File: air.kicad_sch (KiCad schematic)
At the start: 36 parts, among them J1 Conn_01x05, J2 Conn_01x05, J3 Conn_01x04, U1 MT9700, U2 AIR32F103CBT6-LQFP48, U3 RT9013-33GB, U4 USBLC6-2SC6, Y1 8M/20pF

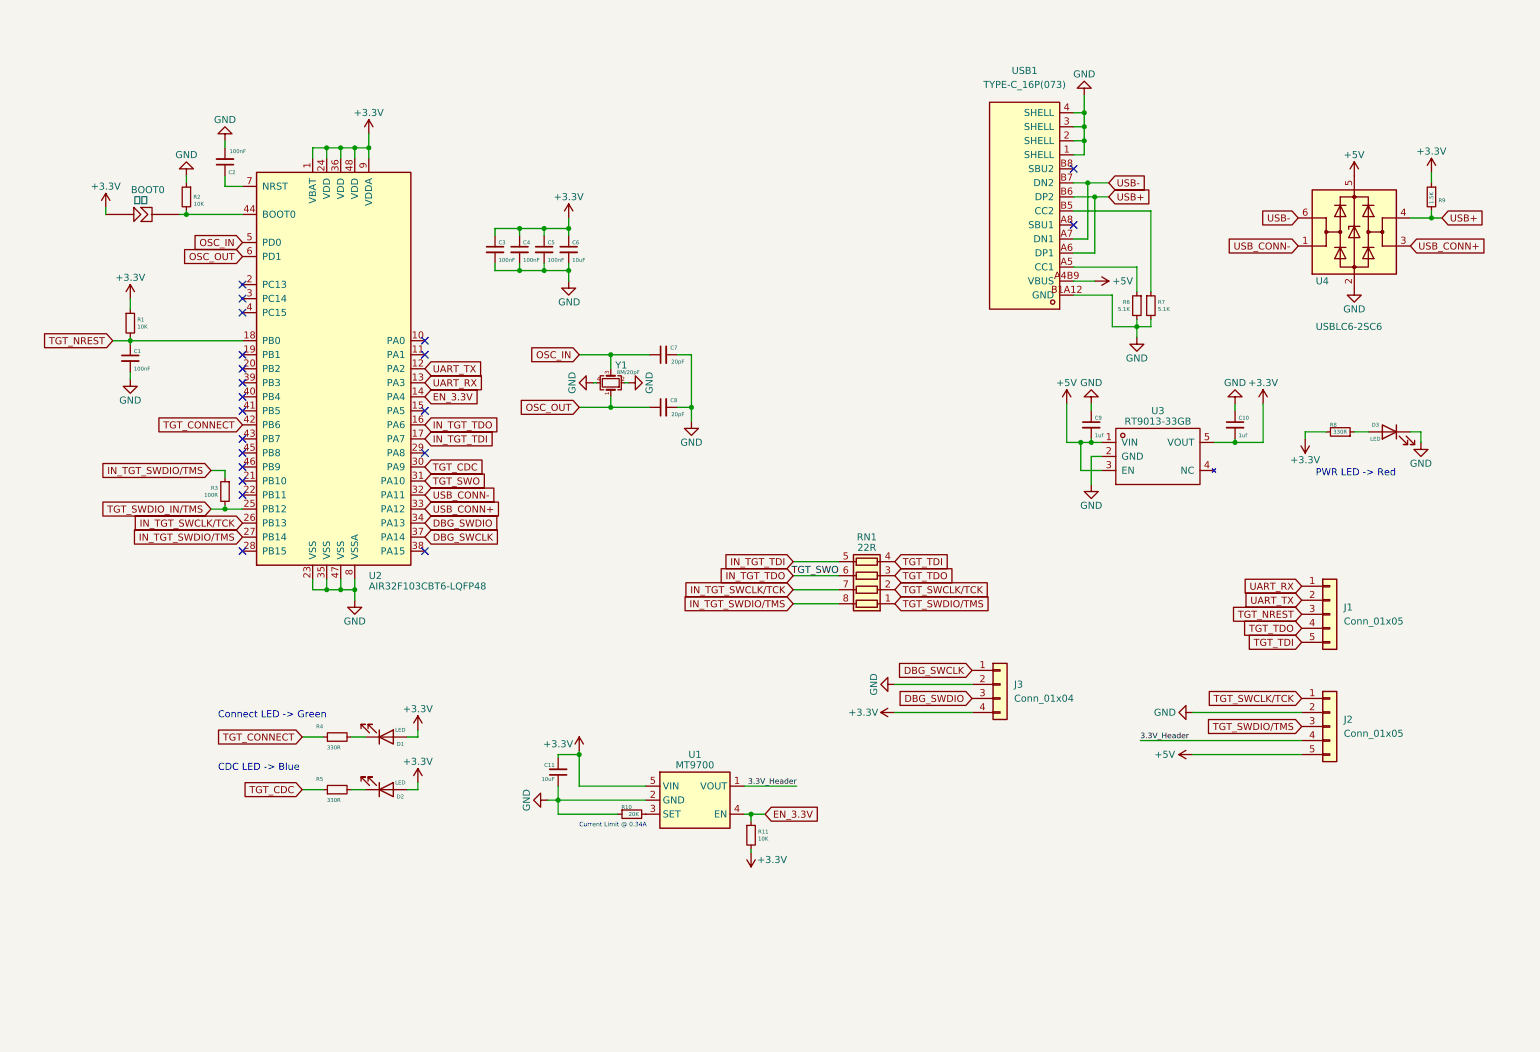
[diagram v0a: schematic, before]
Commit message: still 1.6 but contain some fix to publish work
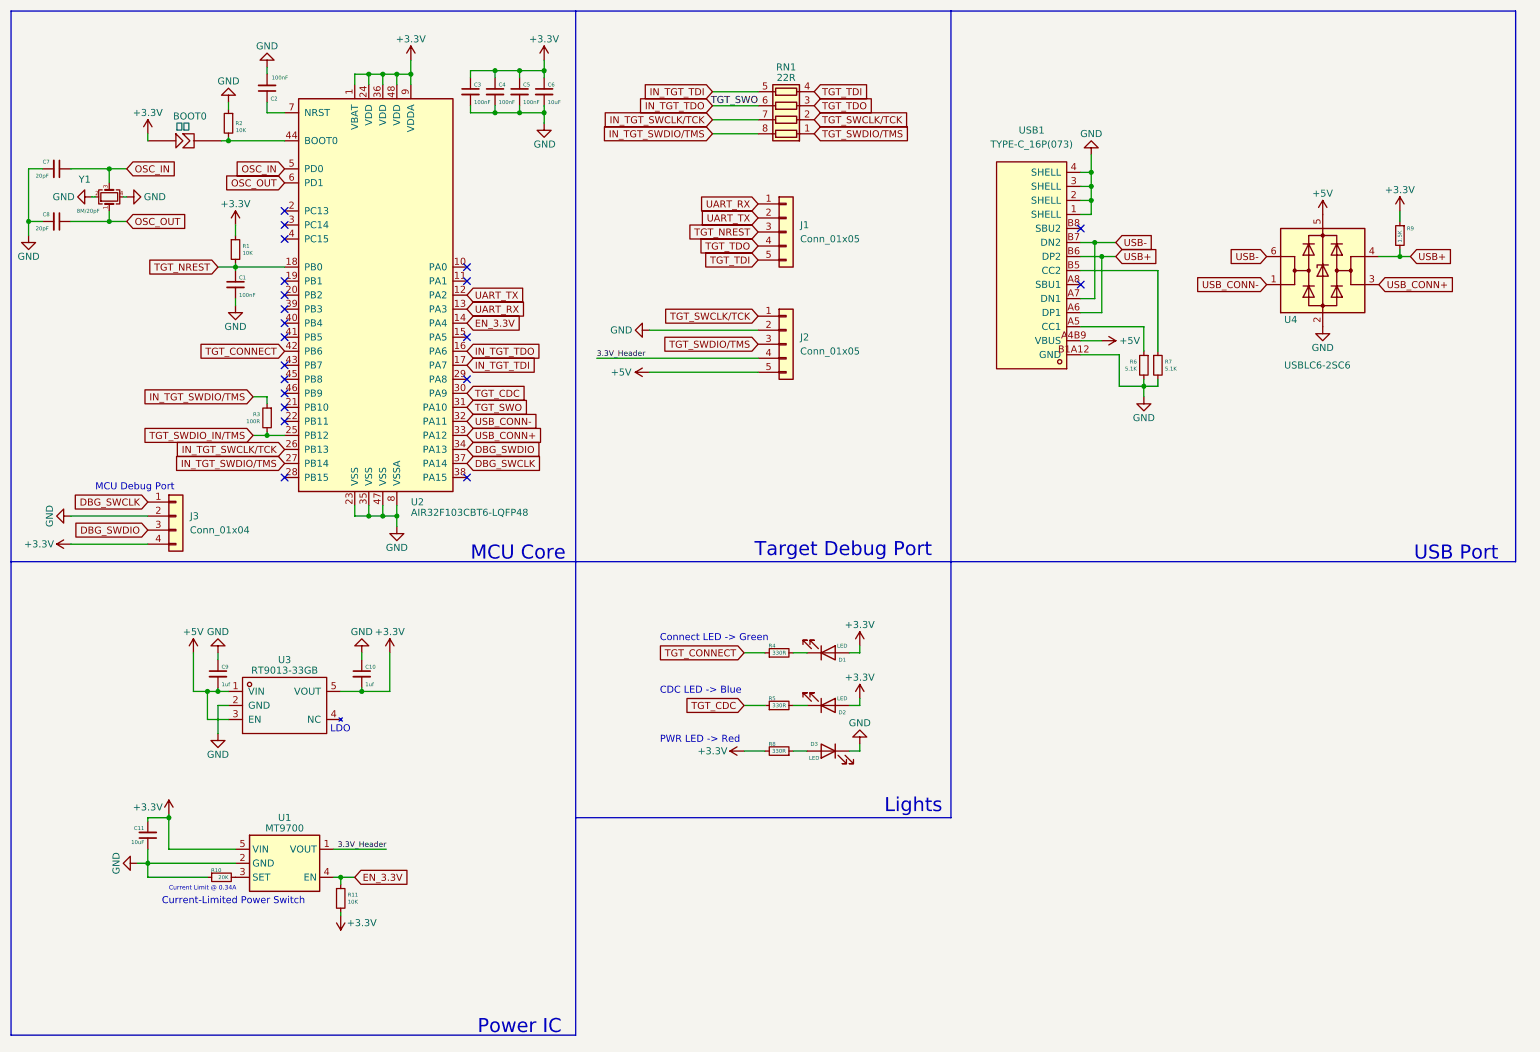
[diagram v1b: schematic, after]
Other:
- note added: "Current-Limited Power Switch"
- note added: "LDO"
- note added: "Lights"
- note added: "MCU Core"
- note added: "MCU Debug Port"
- note added: "Power IC"
- note added: "Target Debug Port"
- note added: "USB Port"
- company: (none) -> [REDACTED]
- title: (none) -> SWD WHISPERER
- moved on the sheet: BOOT0, C1, C10, C11, C2, C3, C4, C5, C6, C7, C8, C9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
